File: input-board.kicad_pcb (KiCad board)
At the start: 2 copper layers, 87.5 x 28.2 mm, 72 parts, among them J1 BTNCON, J12 CAN, J2 BTNCON, J3 SWD, J7 I2C, J8 GAS, J9 BREMSE, SW1 switch-with-led, SW2 switch-with-led, SW3 switch-with-led, SW4 switch-with-led, U1 MPM3620, U2 STM32F103C8Tx, U4 AMS1117-3.3, U7 MCP2542FDxMF, X1 ASCO

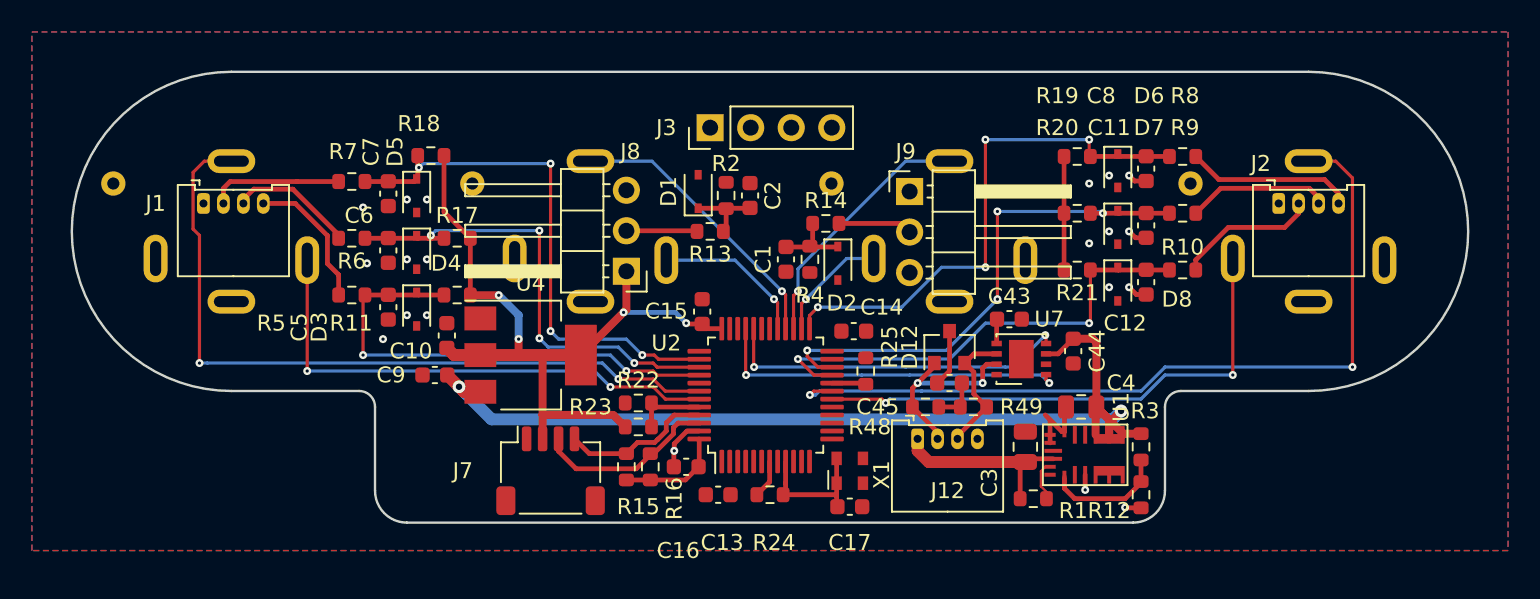
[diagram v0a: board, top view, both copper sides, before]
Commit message: Layout prelim done
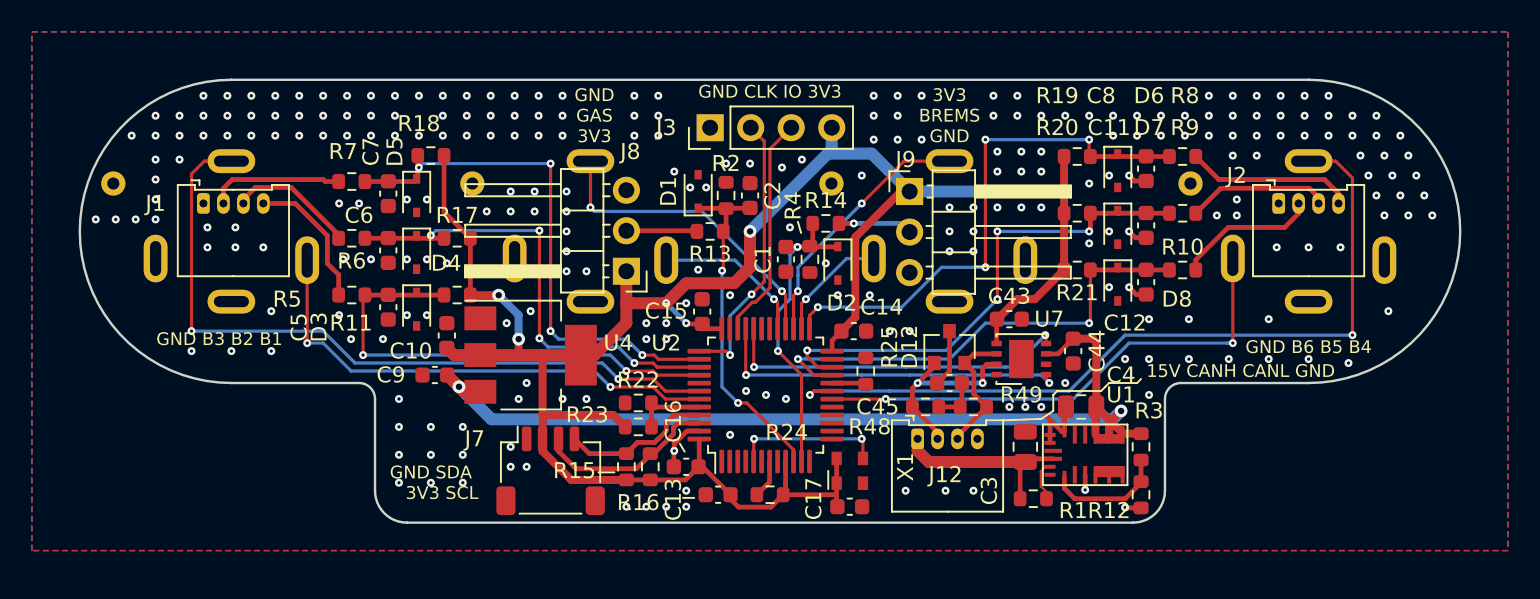
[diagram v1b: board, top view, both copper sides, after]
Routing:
- net +3V3: track 71.6 -> 137.4 mm, vias 4 -> 6
- net SWCLK: track 0.00 -> 17.5 mm, vias 0 -> 2
- net RAW_GAS: track 4.76 -> 21.4 mm, vias 0 -> 2
- net RAW_BREMSE: track 4.76 -> 19.3 mm, vias 0 -> 2
- net SWDIO: track 0.00 -> 14.1 mm
- net Net-(U2-Pad5): track 0.00 -> 9.44 mm, vias 0 -> 2
- net MDLED2: track 17.8 -> 19.7 mm, vias 1 -> 2
- net Net-(U1-Pad4): track 0.00 -> 1.60 mm
- net MDBT4: track 33.2 -> 31.9 mm
- net MDLED4: track 51.2 -> 50.1 mm
- net MDBT1: track 32.2 -> 31.2 mm
- net BTN5: track 32.8 -> 31.8 mm
- net MDLED1: track 46.8 -> 46.1 mm
- net MDLED3: vias 1 -> 2
- net Net-(J9-Pad2): vias 0 -> 1
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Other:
- board size 87.5 x 28.2 mm -> 86.5 x 27.8 mm
- board text added: "15V CANH CANL GND"
- board text added: "3V3 BREMS GND"
- board text added: "GND B3 B2 B1"
- board text added: "GND B6 B5 B4"
- board text added: "GND CLK IO 3V3"
- board text added: "GND GAS 3V3"
- board text added: "GND SDA 3V3 SCL"
